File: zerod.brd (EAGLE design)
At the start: 82.2 x 72.4 mm, 31 parts, among them IC1 NE5532N, IC2 LM3914N

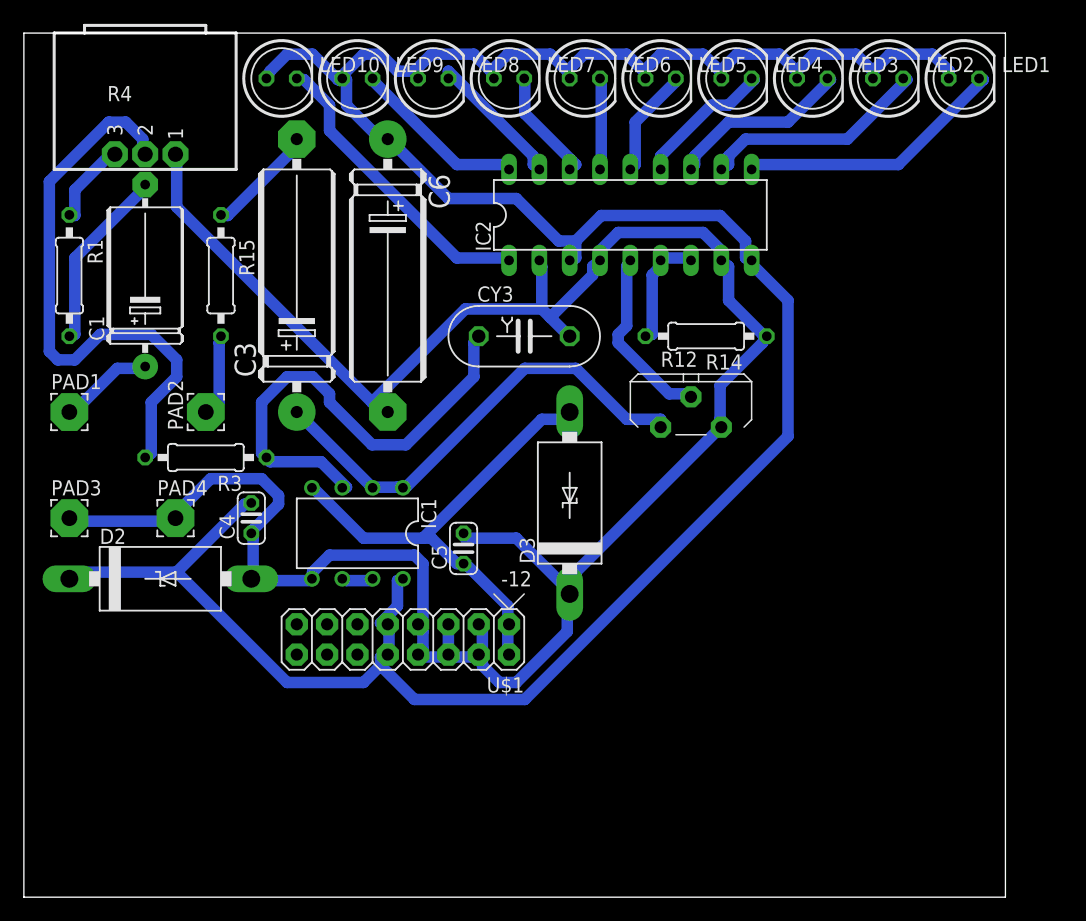
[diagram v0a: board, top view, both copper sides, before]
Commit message: no peak finder and balanced
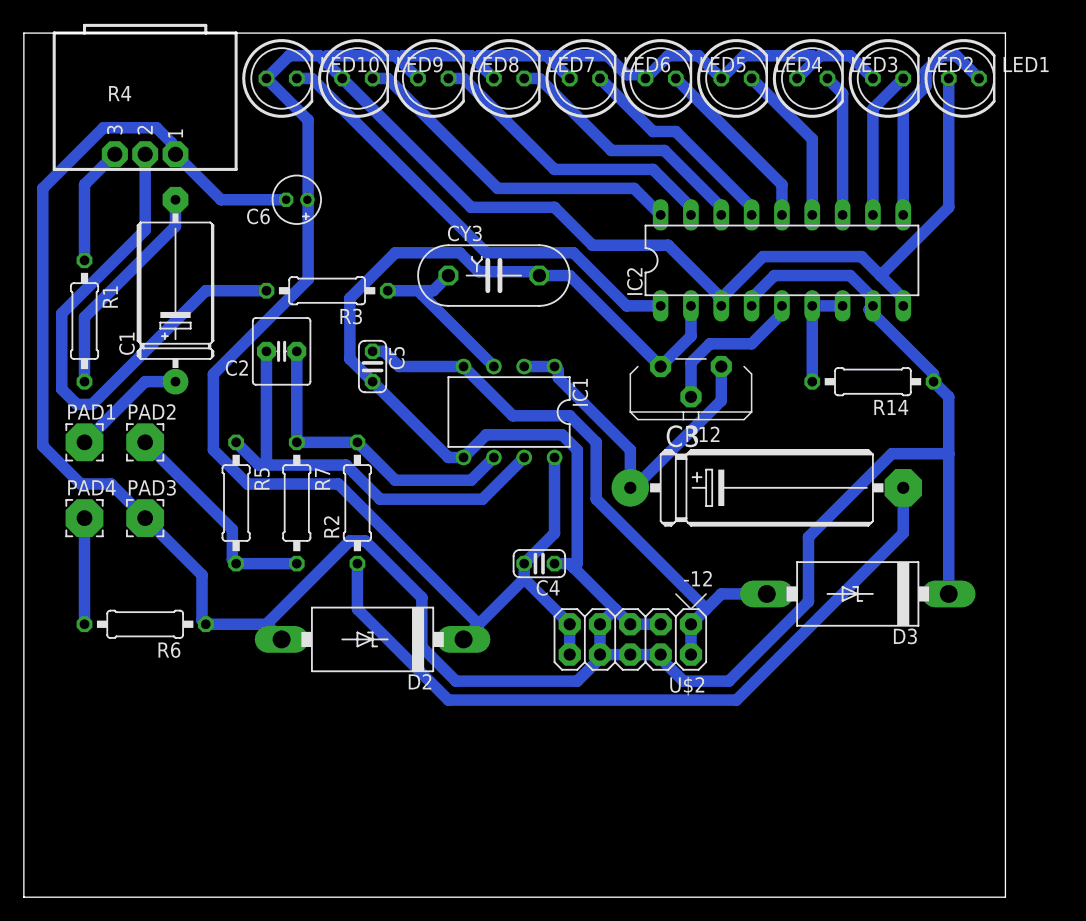
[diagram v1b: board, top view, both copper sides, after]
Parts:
- removed R15: 51, rcl:0207/10
- removed U$1: POWER, eurorack:POWER_16
- added C2: (no value), capacitor-wima:C2.5-6
- added R2, R7: 10k, rcl:0207/10
- added R5, R6: 150, rcl:0207/10
- added U$2: POWER_SIMPLE10, eurorack:POWER_10
- C6: device rcl:E22-6 -> rcl:E1,8-4
- PAD2: value output -> output TIP
- PAD4: value output -> output RING
- moved C3 43.2 mm to (62.2, 41.9), turned to 0 degrees
- moved D3 25.3 mm to (69.8, 33.0), turned to 180 degrees
- moved C4 24.4 mm to (43.2, 35.6), turned to 180 degrees
- moved D2 18.5 mm to (29.2, 29.2), turned to 180 degrees
- moved R3 17.3 mm to (25.4, 58.4)
- moved C5 17.0 mm to (29.2, 52.1), turned to 270 degrees
- moved IC1 16.3 mm to (40.6, 48.3)
- moved R14 14.5 mm to (71.1, 50.8)
- moved IC2 13.3 mm to (63.5, 61.0)
- moved C6 9.92 mm to (22.9, 66.0), turned to 180 degrees
- moved PAD4 7.62 mm to (5.08, 39.4)
- moved PAD3 6.35 mm to (10.2, 39.4)
- moved PAD2 5.68 mm to (10.2, 45.7), turned to 0 degrees
- moved CY3 5.68 mm to (39.4, 59.7)
- moved R1 4.02 mm to (5.08, 55.9)
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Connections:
- removed net N$24: IC1.6, IC1.7
- new net N$15: PAD2.1, R5.2, R7.2
- new net N$5: PAD4.1, R6.2
- new net N$9: C2.2, IC1.7, R5.1
- net +12V: now also U$2.10, U$2.9; no longer U$1.10, U$1.9
- net -12V: now also U$2.1, U$2.2; no longer U$1.1, U$1.2
- net GNDA: now also R6.1, U$2.3, U$2.4, U$2.5, U$2.6, U$2.7, U$2.8; no longer PAD4.1, U$1.3, U$1.4, U$1.5, U$1.6, U$1.7, U$1.8
- net N$3: now also R2.1; no longer R15.1
- net N$8: now also C2.1, IC1.6, R2.2, R7.1; no longer PAD2.1, R15.2
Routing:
- net GNDA: track 199.2 -> 288.4 mm
- net N$3: track 10.2 -> 62.3 mm
- net N$9: track 0.00 -> 37.1 mm
- net N$6: track 40.2 -> 14.5 mm
- net N$8: track 6.98 -> 26.2 mm
- net N$15: track 0.00 -> 18.4 mm
- net N$22: track 14.9 -> 28.9 mm
- net N$21: track 12.0 -> 25.4 mm
- net N$23: track 25.4 -> 38.4 mm
- net N$20: track 9.64 -> 21.6 mm
- net N$10: track 39.7 -> 28.8 mm
- net N$19: track 7.67 -> 17.8 mm
- net N$5: track 0.00 -> 8.89 mm
- net -12V: track 41.5 -> 49.6 mm
- net +12V: track 229.5 -> 236.8 mm
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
